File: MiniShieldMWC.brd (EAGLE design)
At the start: 44.1 x 20.3 mm, 24 parts

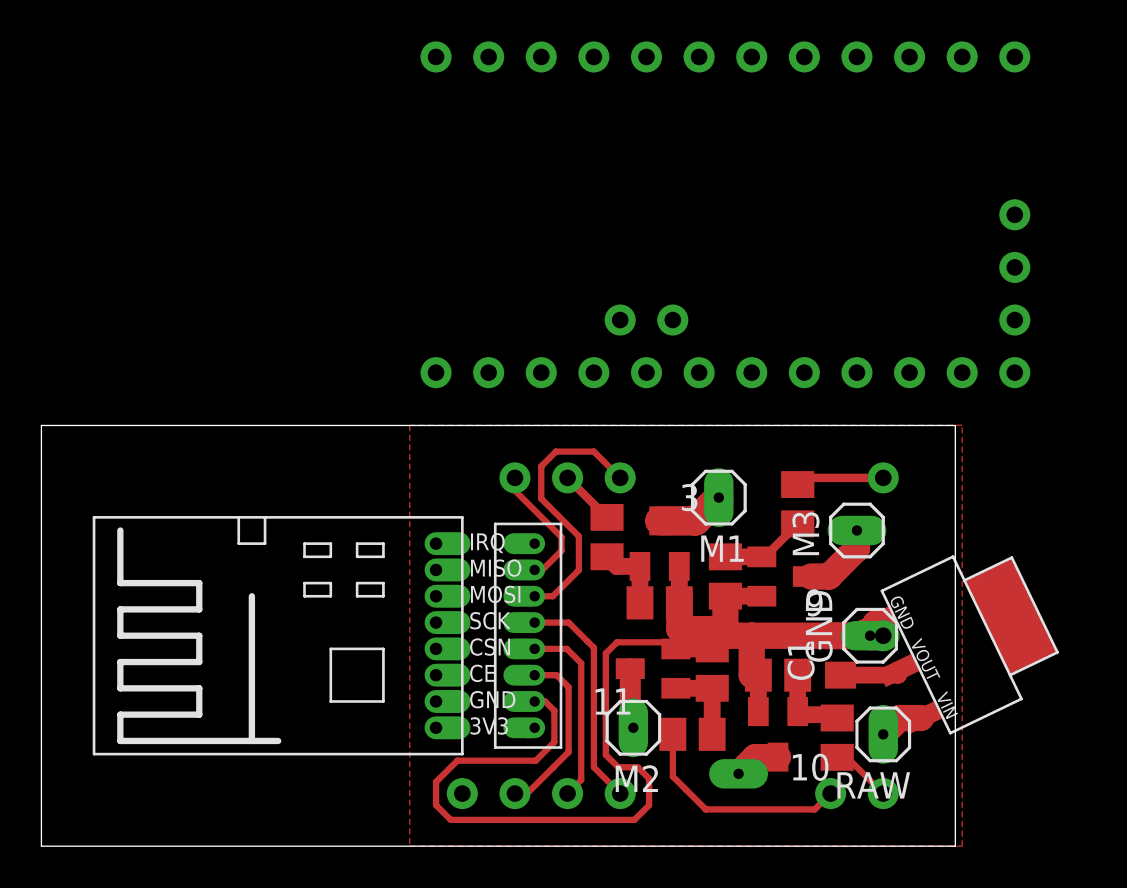
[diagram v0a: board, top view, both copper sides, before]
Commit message: 1.1
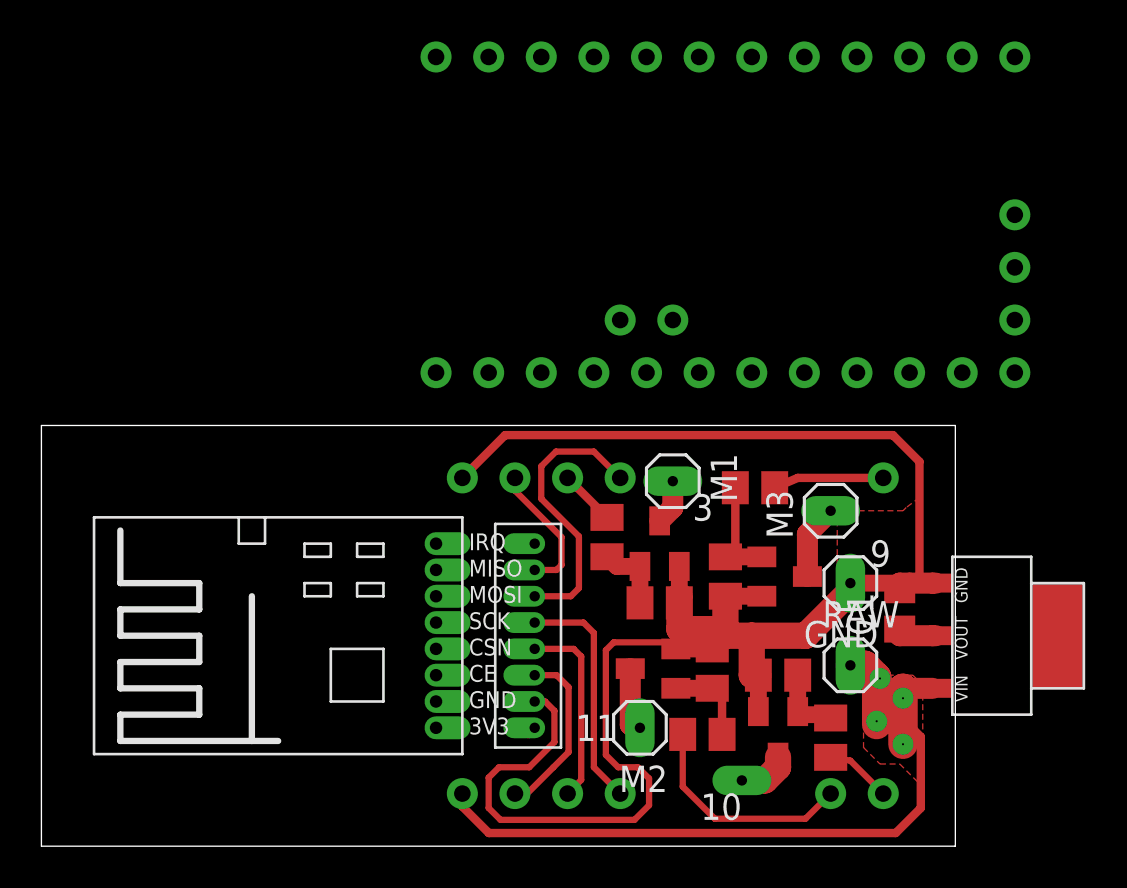
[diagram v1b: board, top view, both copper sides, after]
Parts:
- moved RAW 3.69 mm to (39.1, 8.73), turned to 0 degrees
- moved C1 3.62 mm to (41.4, 11.4)
- moved GND 2.71 mm to (39.1, 12.7), turned to 180 degrees
- moved M1 2.36 mm to (30.5, 17.6), turned to 270 degrees
- moved R3 2.21 mm to (34.4, 17.3), turned to 180 degrees
- moved U$3 2.16 mm to (44.0, 10.2), turned to 270 degrees
- moved M3 1.59 mm to (38.1, 16.2)
- moved R2 0.48 mm to (31.9, 5.40)
- moved M4 0.35 mm to (33.8, 3.17)
- moved M2 0.32 mm to (28.9, 5.71)
- moved R4 0.32 mm to (38.1, 5.24)
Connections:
- net P$1 renamed N$19
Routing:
- net N$19: track 2.16 -> 41.8 mm, vias 0 -> 4
- net GND: track 59.0 -> 87.1 mm
- net N$12: track 3.32 -> 2.18 mm
- net N$3: track 4.48 -> 5.57 mm
- net +3V3: track 3.46 -> 2.51 mm
- net N$7: track 4.45 -> 5.34 mm
- net MOSI: track 13.1 -> 13.6 mm
- added copper zone on layer 1, net GND
- added copper zone on layer 1, net N$19
- removed copper zone on layer 1, net N$14

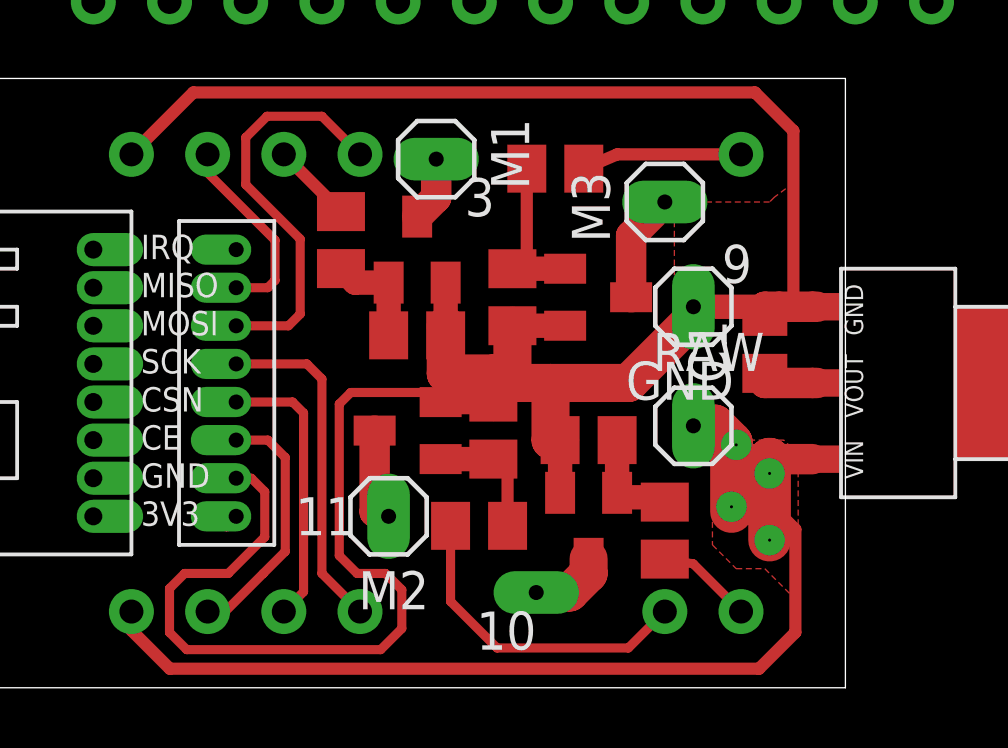
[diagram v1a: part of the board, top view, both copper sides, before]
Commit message: 1.1.1
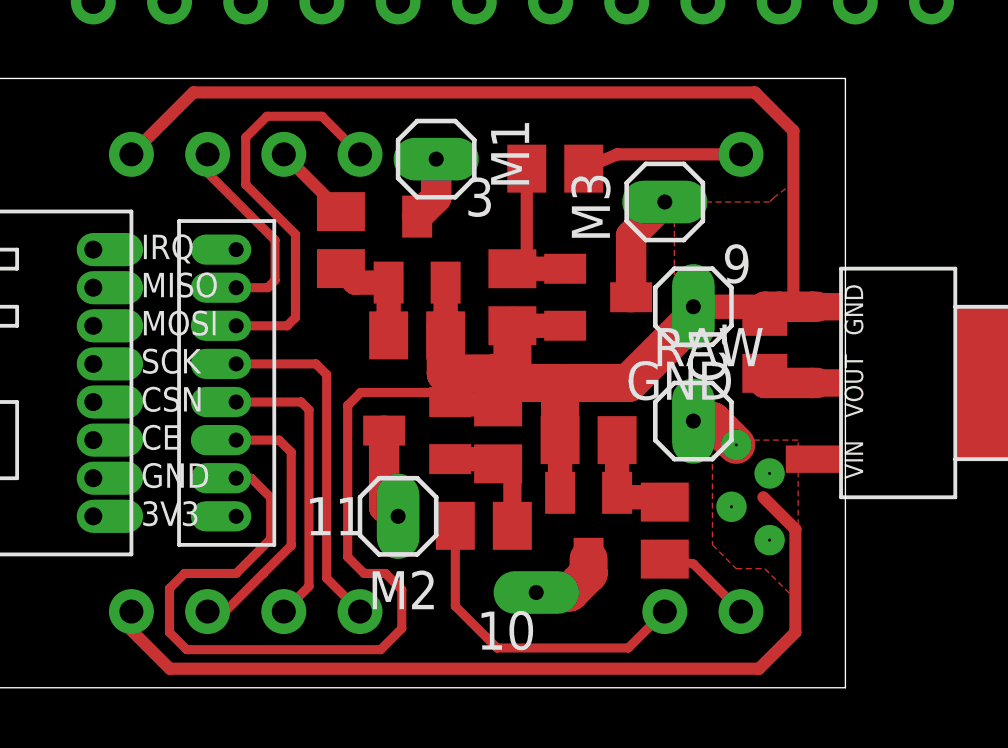
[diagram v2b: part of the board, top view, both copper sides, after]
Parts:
- moved M2 0.32 mm to (29.2, 5.71)
- moved 11 0.32 mm to (29.8, 8.57)
- moved R6 0.22 mm to (32.5, 8.41)
- moved R2 0.16 mm to (32.1, 5.40)
- moved RAW 0.16 mm to (39.1, 8.89)
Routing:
- net N$19: track 41.8 -> 30.5 mm
- net N$2: track 4.46 -> 5.00 mm
